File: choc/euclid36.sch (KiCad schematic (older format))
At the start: 104 parts, among them SW10 SW_PUSH, SW11 SW_PUSH, SW12 SW_PUSH, SW14 SW_PUSH, SW15 SW_PUSH, SW16 SW_PUSH, SW17 SW_PUSH, SW18 SW_PUSH, SW19 SW_PUSH, SW2 SW_PUSH, SW20 SW_PUSH, SW21 SW_PUSH, SW22 SW_PUSH, SW23 SW_PUSH, SW25 SW_PUSH, SW26 SW_PUSH, SW27 SW_PUSH, SW28 SW_PUSH, SW29 SW_PUSH, SW3 SW_PUSH, SW31 SW_PUSH, SW32 SW_PUSH, SW33 SW_PUSH, SW34 SW_PUSH, SW35 SW_PUSH, SW37 SW_PUSH, SW38 SW_PUSH, SW39 SW_PUSH, SW4 SW_PUSH, SW40 SW_PUSH, SW41 SW_PUSH, SW42 SW_PUSH, SW5 SW_PUSH, SW6 SW_PUSH, SW8 SW_PUSH, SW9 SW_PUSH, U2 ATmega32U4-MU, Y1 XTAL

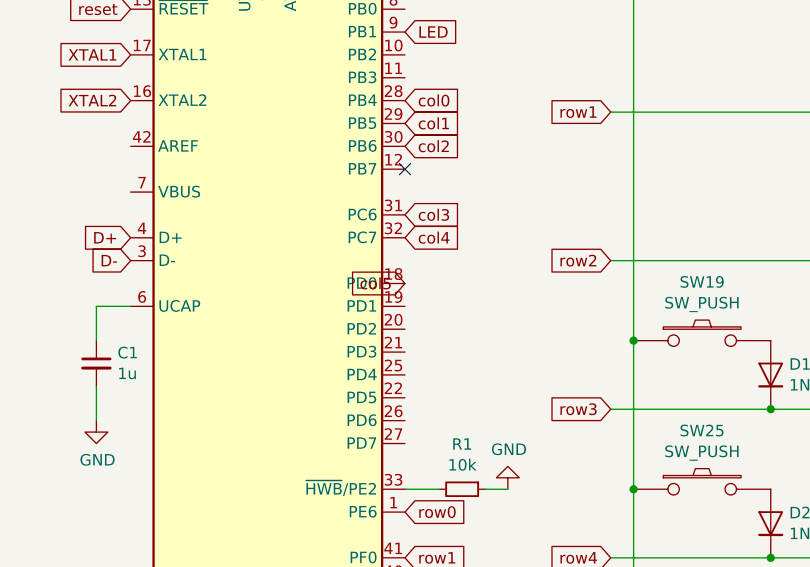
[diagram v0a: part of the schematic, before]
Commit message: Small fixes
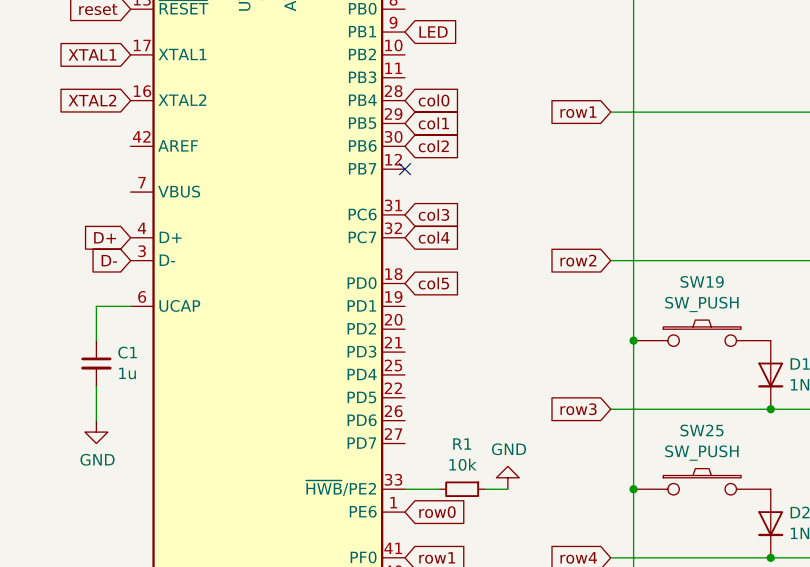
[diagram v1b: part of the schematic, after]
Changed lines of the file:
@@
 Text GLabel 2300 2850 2    50   Input ~ 0
 col4
-Text GLabel 2300 3050 0    50   Input ~ 0
+Text GLabel 2300 3050 2    50   Input ~ 0
 col5
 Text GLabel 2300 4050 2    50   Input ~ 0
